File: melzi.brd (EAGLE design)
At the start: 208.3 x 49.5 mm, 121 parts, among them IC5 7805DT, IC6 ATMEGA1284P, IC7 4050D, IC8 FT232RL-BASICSSOP, M1 RFP30N06LE, M2 RFP30N06LE, M3 RFP30N06LE, Q1 16MHZ, U1 A4982, U2 A4982, U3 A4982, U4 A4982, X1 MICROSD, X2 MINI-USB-SHIELD-UX60-MB-5ST

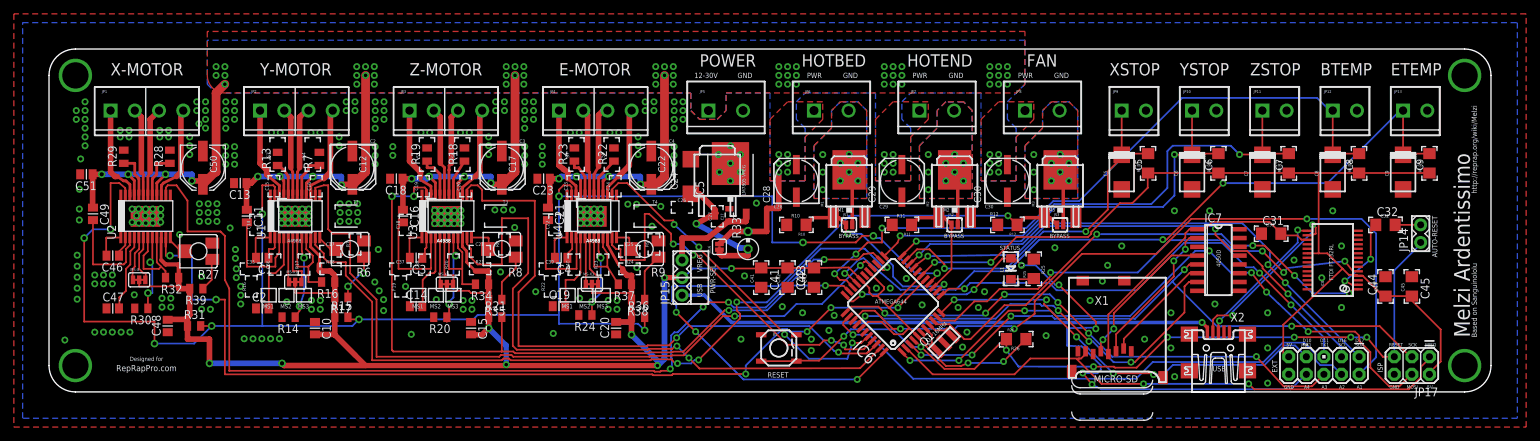
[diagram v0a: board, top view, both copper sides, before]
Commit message: Melzi 2.0 finished (e&oe...)
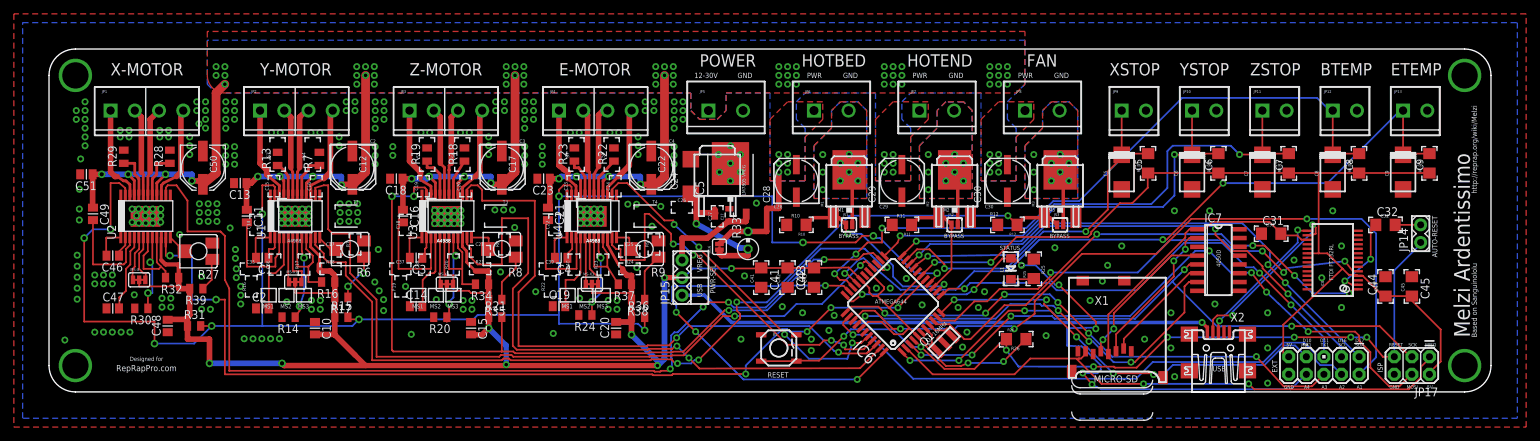
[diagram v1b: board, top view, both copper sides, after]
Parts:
- JP4: value Y-MOT -> E-MOT
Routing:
- net N$7: track 2.16 -> 3.60 mm
- net VMOT: track 191.8 -> 192.4 mm
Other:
- board text added: "+"
- board text added: "-"
- board text added: "E motor"
- board text added: "X motor"
- board text added: "Y motor"
- board text added: "Z motor"
- board text added: "bed"
- board text added: "btemp"
- board text added: "etemp"
- board text added: "fan"
- board text added: "hot end"
- board text added: "power"
- board text added: "reprappro.com RepRap Melzi V2.0 Licence: GPL"
- board text added: "x-stop"
- board text added: "y-stop"
- board text added: "z-stop"
